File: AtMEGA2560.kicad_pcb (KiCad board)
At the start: 4 copper layers, 101.6 x 53.3 mm, 60 parts, among them IC1 NCP1117-5.0_SOT223, IC3 ATmega2560-16AU, IC4 ATmega16U2-AU, IC6 LP2985-3.3, IC7 LMV358IDGKR, T1 FDN340P, X1 DC21MMX, X2 USB-B_TH, Y1 CSTCE16M0V53-R0 16MHZ, Y2 16MHz

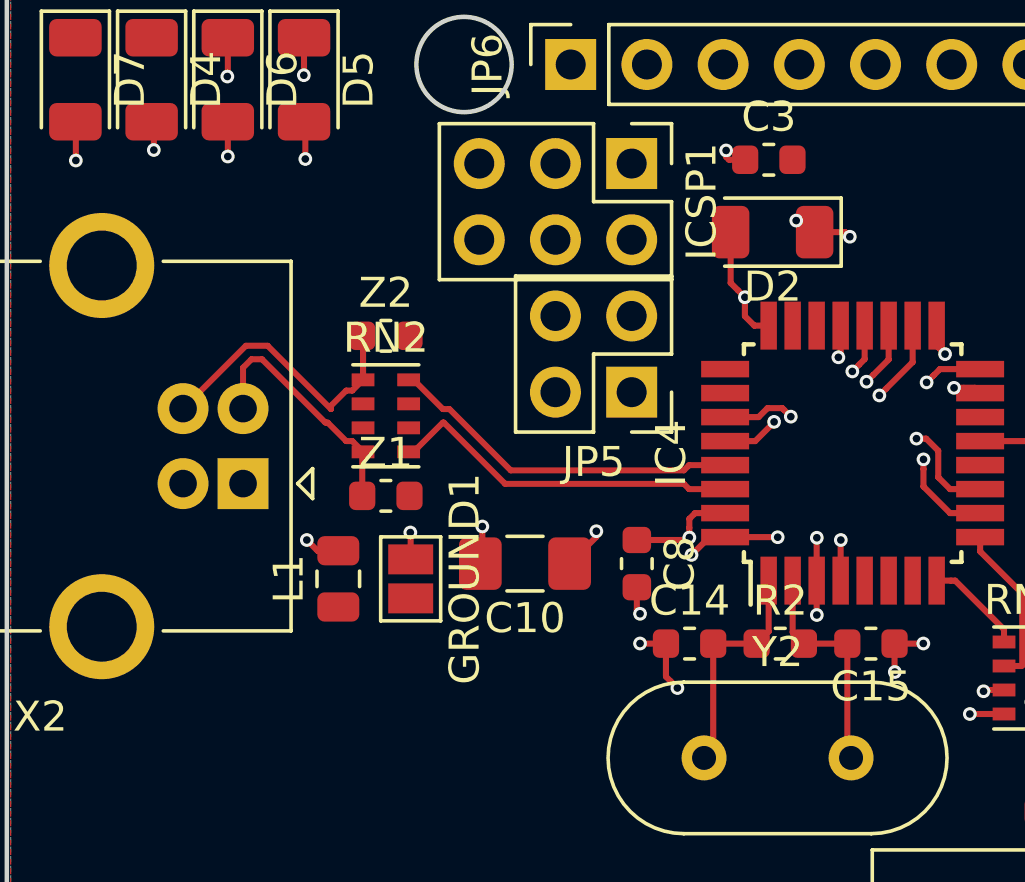
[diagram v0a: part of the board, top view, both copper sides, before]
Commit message: Initial USB floods
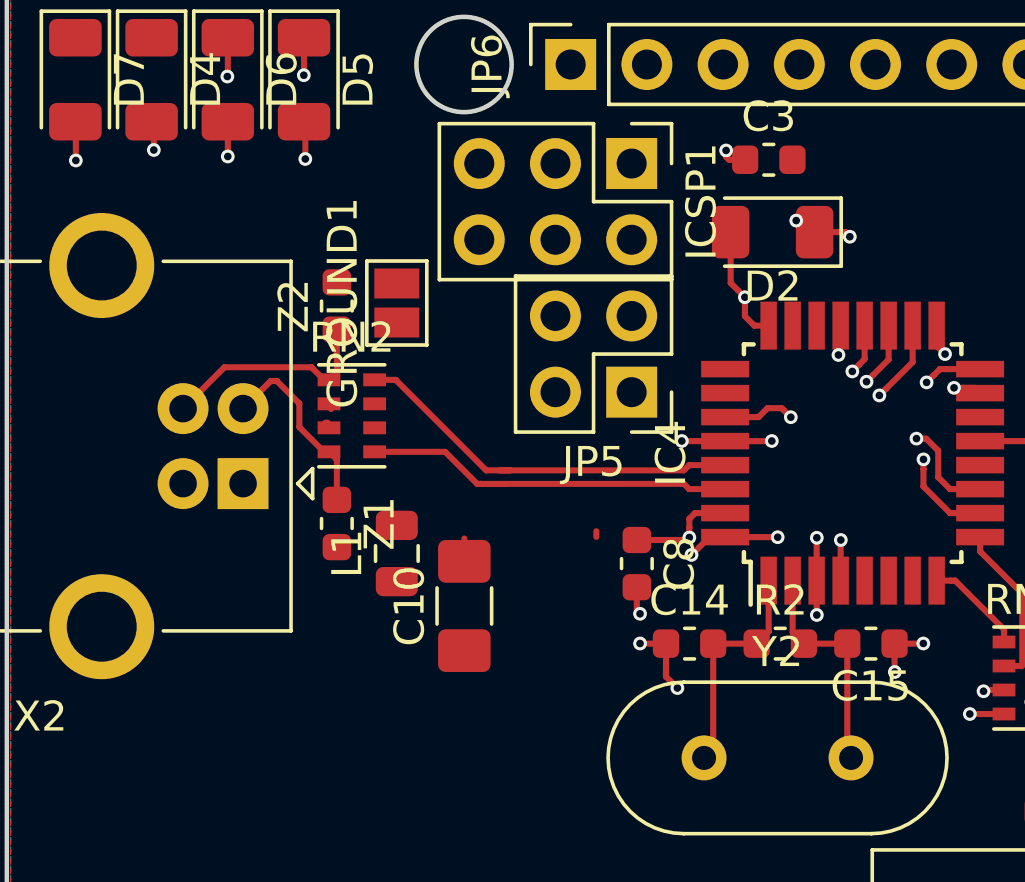
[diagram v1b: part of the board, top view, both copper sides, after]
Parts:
- moved GROUND1 9.21 mm to (89.2, 79.1), turned to 90 degrees
- moved C10 2.47 mm to (91.5, 89.2), turned to 90 degrees
- moved L1 2.13 mm to (89.2, 87.4)
- moved Z2 1.91 mm to (87.2, 79.2), turned to 90 degrees
- moved Z1 1.88 mm to (87.2, 86.4), turned to 270 degrees
- moved RN2 1.13 mm to (87.7, 82.8)
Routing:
- net /VBUS: track 29.9 -> 1.09 mm
- net /USBGND: track 29.7 -> 3.86 mm, vias 4 -> 2
- net /USB2+: track 9.69 -> 7.39 mm
- net Net-(D5-Pad2): track 36.8 -> 34.9 mm
- net /USB2-: track 8.24 -> 6.39 mm
- net /USB1+: track 11.9 -> 13.4 mm
- net Net-(C10-Pad1): track 12.1 -> 10.7 mm, vias 2 -> 1
- net Net-(D6-Pad2): track 39.3 -> 38.1 mm
- added copper zone on In1.Cu, net /USBGND
- added copper zone on In1.Cu, net /USBSHIELD
- removed copper zone on In1.Cu, net GND
